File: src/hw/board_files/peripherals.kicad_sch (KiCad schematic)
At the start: 35 parts, among them J3 Screw_Terminal_01x03, J4 Molex 104031-0811, Q1 PMOS, U4 NEO-M9N, U5 BQ27411DRZT-G1A, U6 SHT30-DIS

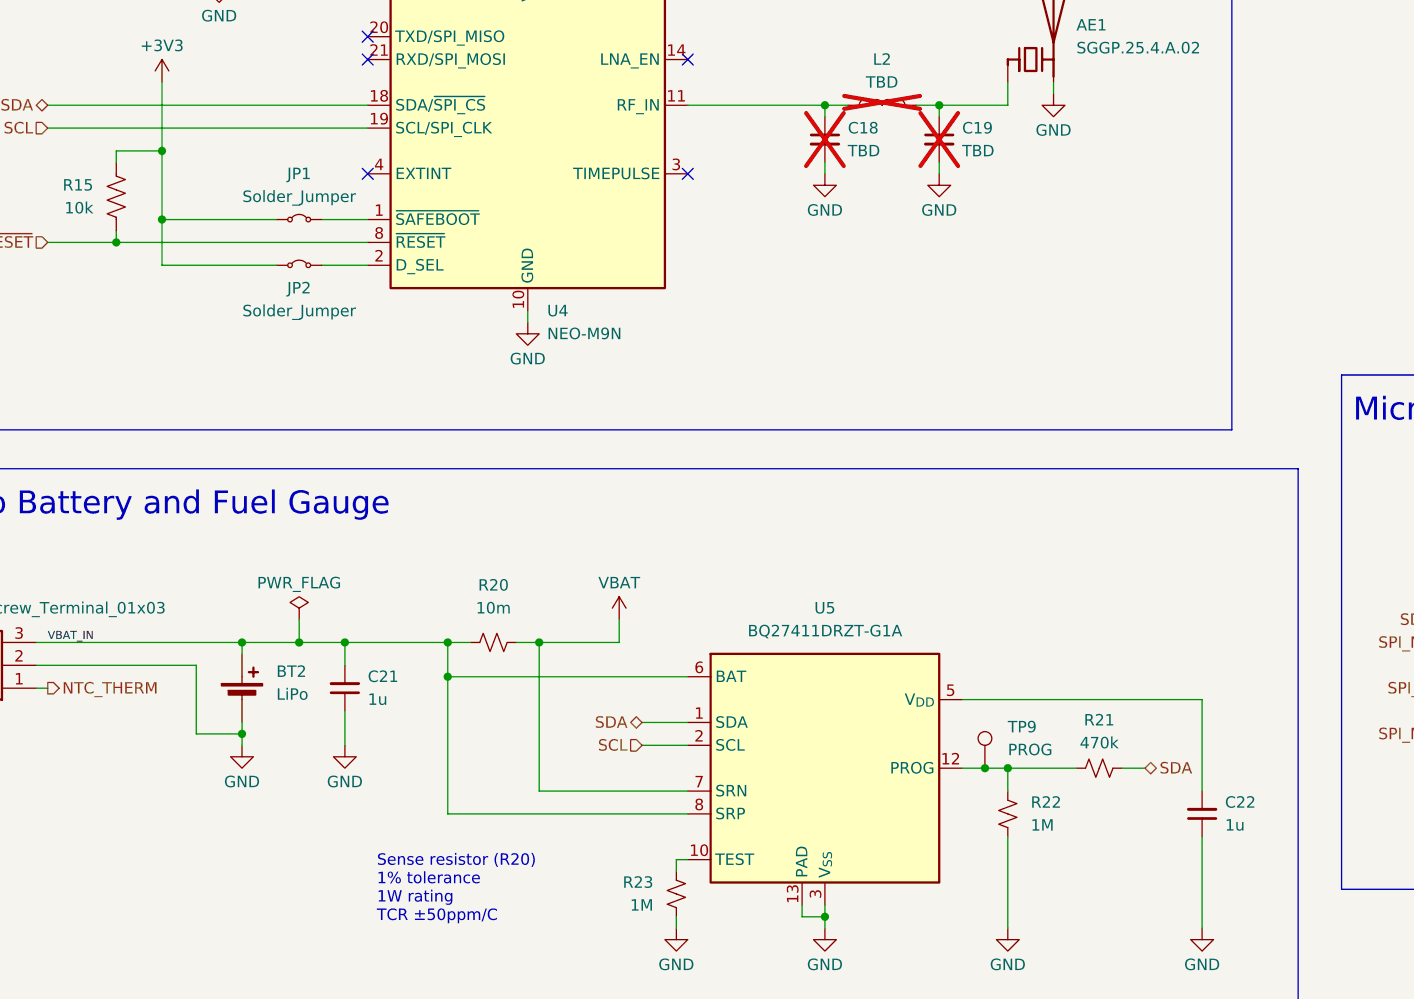
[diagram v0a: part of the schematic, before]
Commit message: Layout progress
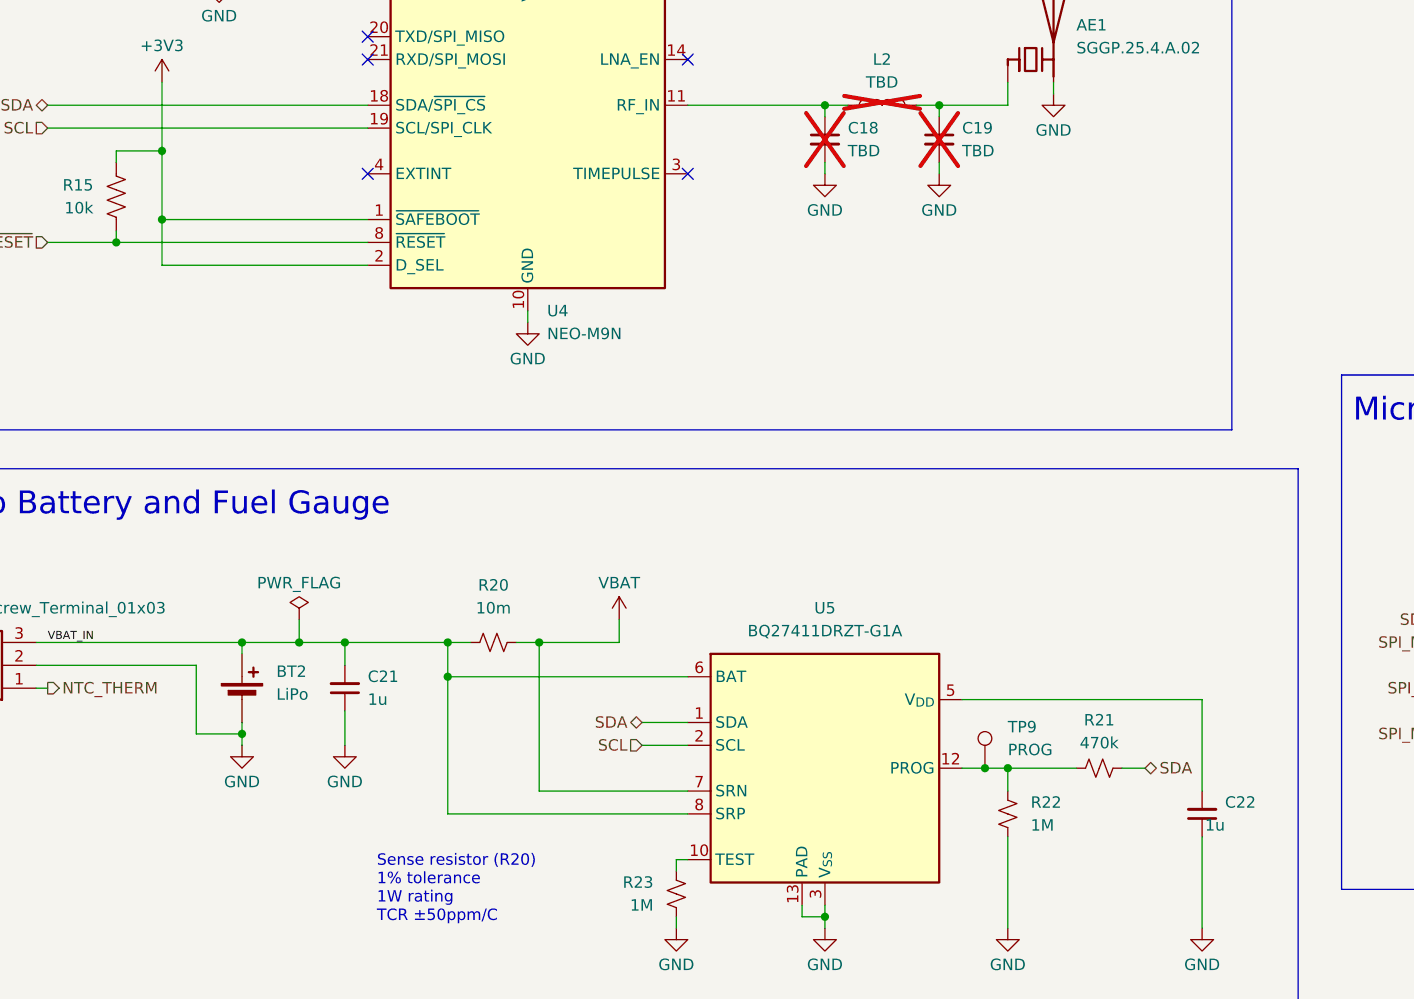
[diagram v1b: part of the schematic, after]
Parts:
- removed JP1, JP2: Solder_Jumper, Jumper:SolderJumper-2_P1.3mm_Open_TrianglePad1.0x1.5mm, symbol Jumper:Jumper_2_Small_Bridged
- TP8, TP9: footprint TestPoint:TestPoint_Pad_D1.5mm -> TestPoint:TestPoint_Pad_D1.0mm
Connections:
- net +3V3: now also U4.1 (~{SAFEBOOT}), U4.2 (D_SEL)
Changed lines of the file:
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@@
 	(wire
 		(pts
-			(xy 40.64 86.36) (xy 53.34 86.36)
+			(xy 40.64 86.36) (xy 63.5 86.36)
 		)
 		(stroke
@@
 	(wire
 		(pts
-			(xy 58.42 86.36) (xy 63.5 86.36)
-		)
-		(stroke
-			(width 0)
-			(type default)
-		)
-	)
-	(wire
-		(pts
-			(xy 58.42 91.44) (xy 63.5 91.44)
-		)
-		(stroke
-			(width 0)
-			(type default)
-		)
-	)
-	(wire
-		(pts
 			(xy 27.94 138.43) (xy 26.67 138.43)
 		)
@@
 	(wire
 		(pts
-			(xy 40.64 91.44) (xy 53.34 91.44)
+			(xy 40.64 91.44) (xy 63.5 91.44)
 		)
 		(stroke
@@
 			)
 		)
-		(property "Footprint" "TestPoint:TestPoint_Pad_D1.5mm"
+		(property "Footprint" "TestPoint:TestPoint_Pad_D1.0mm"
 			(at 137.16 147.32 0)
 			(effects
@@
 	)
 	(symbol
-		(lib_id "Jumper:Jumper_2_Small_Bridged")
-		(at 55.88 91.44 0)
-		(unit 1)
-		(exclude_from_sim no)
-		(in_bom yes)
-		(on_board yes)
-		(dnp no)
-		(fields_autoplaced yes)
-		(property "Reference" "JP2"
-			(at 55.88 93.98 0)
-			(effects
-				(font
-					(size 1.27 1.27)
-				)
-			)
-		)
-		(property "Value" "Solder_Jumper"
-			(at 55.88 96.52 0)
-			(effects
-				(font
-					(size 1.27 1.27)
-				)
-			)
-		)
-		(property "Footprint" "Jumper:SolderJumper-2_P1.3mm_Open_TrianglePad1.0x1.5mm"
-			(at 55.88 91.44 0)
-			(effects
-				(font
-					(size 1.27 1.27)
-				)
-				(hide yes)
-			)
-		)
-		(property "Datasheet" "~"
-			(at 55.88 91.44 0)
-			(effects
-				(font
-					(size 1.27 1.27)
-				)
-				(hide yes)
-			)
-		)
-		(property "Description" "Jumper, 2-pole, small symbol, bridged"
-			(at 55.88 91.44 0)
-			(effects
-				(font
-					(size 1.27 1.27)
-				)
-				(hide yes)
-			)
-		)
-		(pin "1"
-		)
-		(pin "2"
-		)
-		(instances
-			(project ""
-				(path "/2c77a8ba-b277-4959-adec-d3fc778c7960/81382524-b053-4c3c-9e13-c8b314c52639"
-					(reference "JP2")
-					(unit 1)
-				)
-			)
-		)
-	)
-	(symbol
 		(lib_id "Device:R_Small_US")
 		(at 144.78 147.32 270)
@@
 		(on_board yes)
 		(dnp no)
-		(fields_autoplaced yes)
 		(property "Reference" "C22"
 			(at 158.75 151.1235 0)
@@
 					(size 1.27 1.27)
 				)
-				(justify right)
+				(justify left)
 			)
 		)
@@
 	)
 	(symbol
-		(lib_id "Jumper:Jumper_2_Small_Bridged")
-		(at 55.88 86.36 0)
-		(unit 1)
-		(exclude_from_sim no)
-		(in_bom yes)
-		(on_board yes)
-		(dnp no)
-		(property "Reference" "JP1"
-			(at 55.88 81.28 0)
-			(effects
-				(font
-					(size 1.27 1.27)
-				)
-			)
-		)
-		(property "Value" "Solder_Jumper"
-			(at 55.88 83.82 0)
-			(effects
-				(font
-					(size 1.27 1.27)
-				)
-			)
-		)
-		(property "Footprint" "Jumper:SolderJumper-2_P1.3mm_Open_TrianglePad1.0x1.5mm"
-			(at 55.88 86.36 0)
-			(effects
-				(font
-					(size 1.27 1.27)
-				)
-				(hide yes)
-			)
-		)
-		(property "Datasheet" "~"
-			(at 55.88 86.36 0)
-			(effects
-				(font
-					(size 1.27 1.27)
-				)
-				(hide yes)
-			)
-		)
-		(property "Description" "Jumper, 2-pole, small symbol, bridged"
-			(at 55.88 86.36 0)
-			(effects
-				(font
-					(size 1.27 1.27)
-				)
-				(hide yes)
-			)
-		)
-		(pin "1"
-		)
-		(pin "2"
-		)
-		(instances
-			(project "pocket-caddy"
-				(path "/2c77a8ba-b277-4959-adec-d3fc778c7960/81382524-b053-4c3c-9e13-c8b314c52639"
-					(reference "JP1")
-					(unit 1)
-				)
-			)
-		)
-	)
-	(symbol
 		(lib_id "Device:R_Small_US")
 		(at 134.62 152.4 180)
@@
 			)
 		)
-		(property "Footprint" "TestPoint:TestPoint_Pad_D1.5mm"
+		(property "Footprint" "TestPoint:TestPoint_Pad_D1.0mm"
 			(at 250.19 44.45 0)
 			(effects
